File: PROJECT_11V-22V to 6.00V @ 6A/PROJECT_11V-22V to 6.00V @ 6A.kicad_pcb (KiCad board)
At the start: 2 copper layers, 33.1 x 21.4 mm, 21 parts, among them IC1 TPS56A37RPAR, J1 Screw_Terminal_01x02, J2 Screw_Terminal_01x02

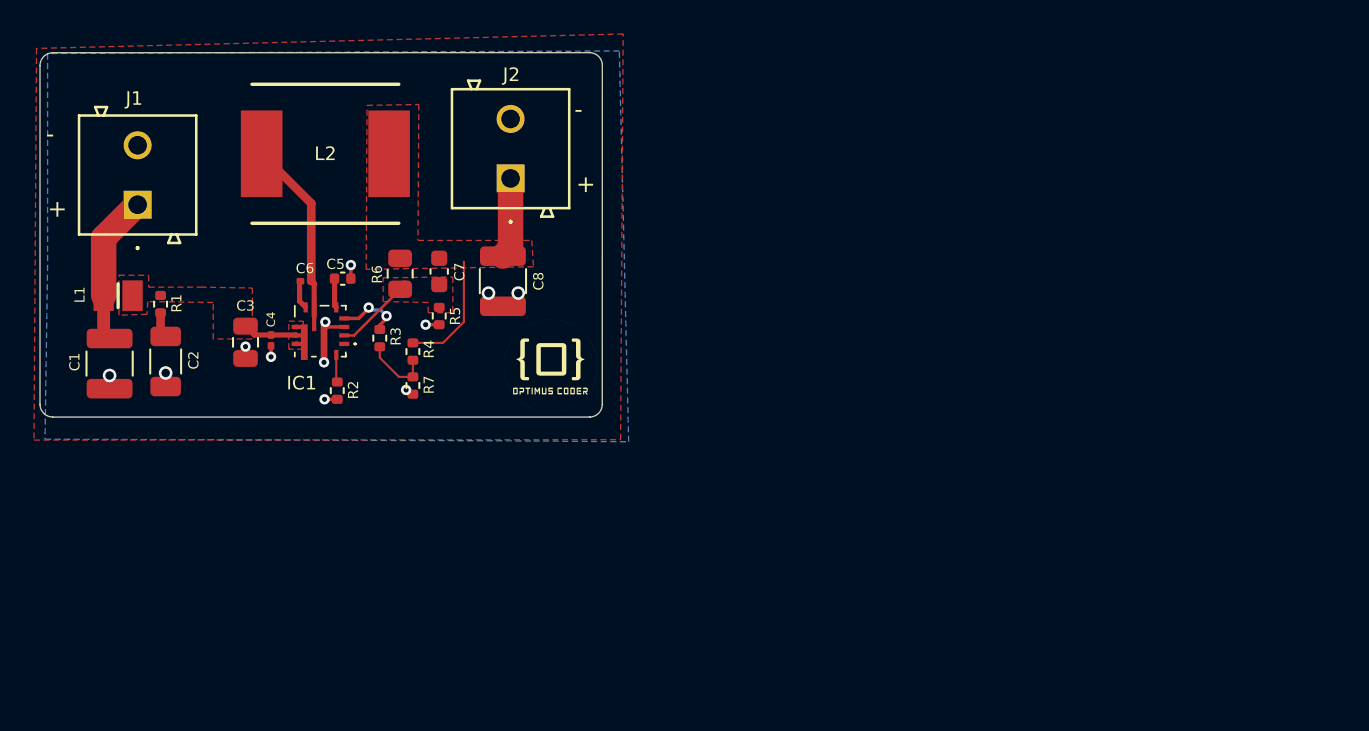
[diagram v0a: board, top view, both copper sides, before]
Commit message: Add files via upload
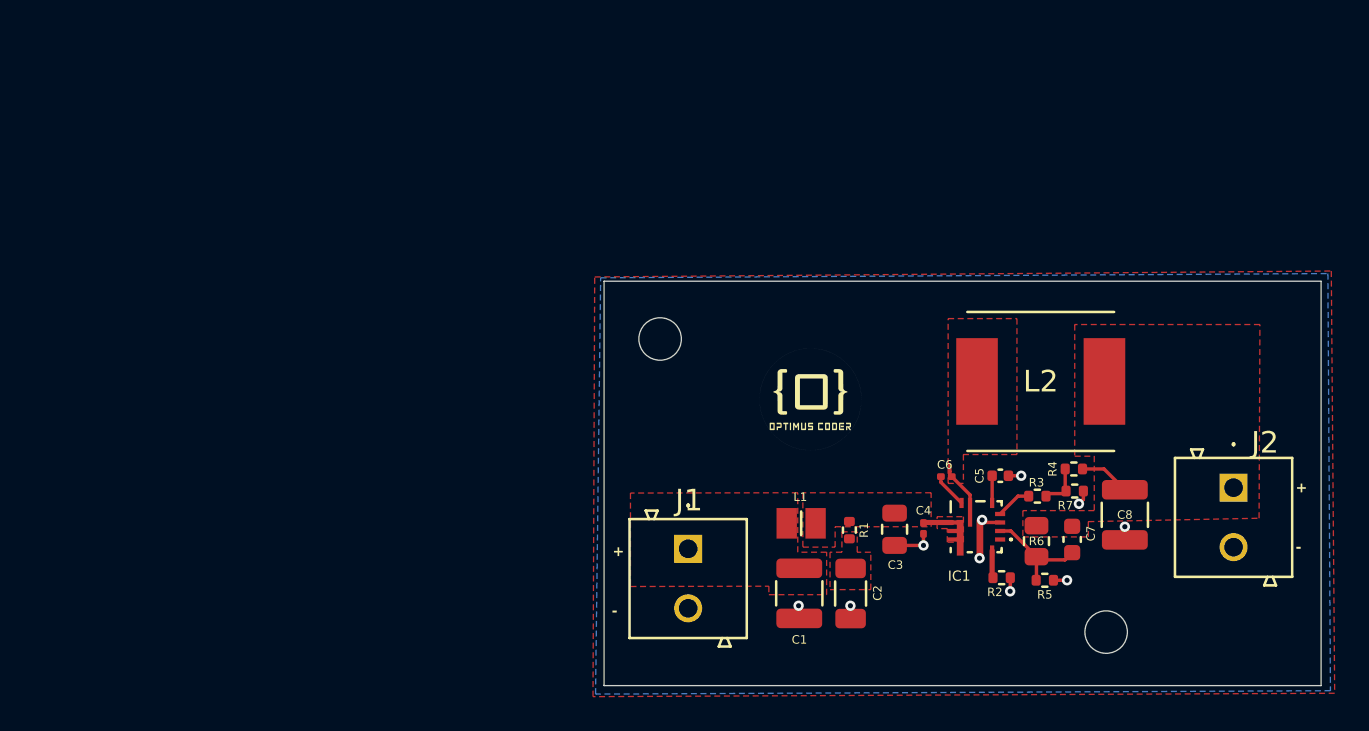
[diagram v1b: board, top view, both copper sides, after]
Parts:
- added REF**: MountingHole_2.5mm, MountingHole:MountingHole_2.5mm, F.Cu at (87.4, 107.0)
- added REF**: MountingHole_2.5mm, MountingHole:MountingHole_2.5mm, F.Cu at (113.7, 124.3)
- moved J2 46.3 mm to (121.2, 115.8), turned to -90 degrees
- moved L2 44.2 mm to (109.8, 109.5)
- moved C1 42.8 mm to (95.6, 122.0)
- moved R1 42.7 mm to (98.5, 118.3)
- moved C2 42.6 mm to (98.6, 122.0)
- moved L1 42.4 mm to (95.7, 117.9)
- moved R6 40.6 mm to (109.5, 119.0)
- moved R2 40.6 mm to (107.5, 121.1), turned to 0 degrees
- moved C7 40.5 mm to (111.7, 118.8)
- moved C5 40.4 mm to (107.4, 115.1)
- moved IC1 40.3 mm to (106.0, 118.1)
- moved C4 40.0 mm to (102.9, 118.2)
- moved R3 39.8 mm to (109.6, 116.3), turned to 0 degrees
- moved C3 39.8 mm to (101.2, 118.2)
- moved R4 39.5 mm to (111.8, 114.7), turned to 0 degrees
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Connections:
- net Net-(C2-Pad1) renamed /Net_C2-R1
- net Net-(IC1-MODE) renamed /MODE
- net Net-(IC1-SS) renamed /SS
- net Net-(IC1-SW) renamed /C6-L2
- net Net-(J1-Pin_1) renamed /V_unfiltered
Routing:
- net /PWR_OUT+: track 12.6 -> 3.00 mm
- net /V_unfiltered: track 8.88 -> 0.00 mm
- net /C6-L2: track 11.0 -> 3.29 mm
- net GND: track 11.1 -> 7.78 mm, vias 12 -> 10
- net /V_filtered: track 4.71 -> 1.70 mm
- net Net-(IC1-PG): track 3.95 -> 2.11 mm, vias 2 -> 0
- net /FB: track 4.80 -> 6.52 mm
- net /Net_C2-R1: track 1.51 -> 0.00 mm
- net +5V: track 4.04 -> 2.62 mm
- added copper zone on F.Cu, net /C6-L2
- added copper zone on F.Cu, net /Net_C2-R1
- added copper zone on F.Cu, net /V_unfiltered
- removed copper zone on F.Cu, net /FB
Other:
- board size 33.1 x 21.4 mm -> 42.2 x 23.8 mm
